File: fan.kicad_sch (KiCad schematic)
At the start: 9 parts, among them J4 Conn_01x04, Q1 BSS138

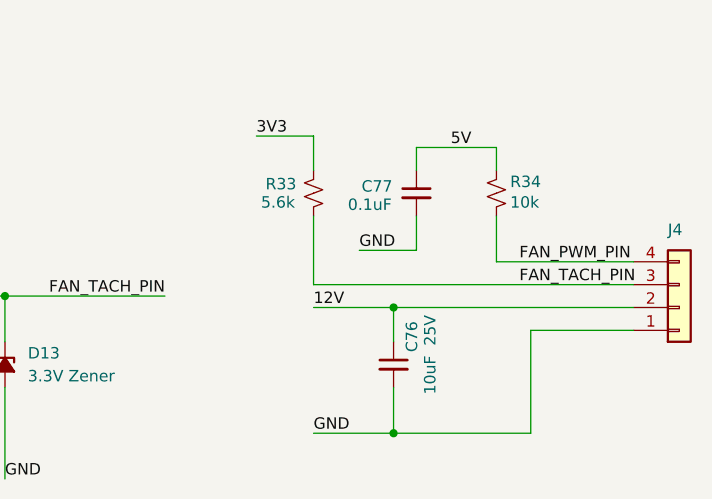
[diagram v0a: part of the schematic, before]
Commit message: run through ERC
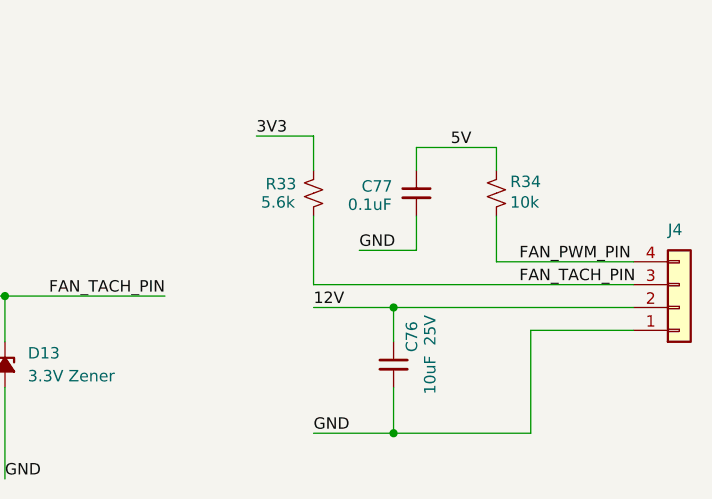
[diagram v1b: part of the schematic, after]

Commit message: adding jlcpcb deets
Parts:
- Q1: FT Rotation Offset (none) -> 180
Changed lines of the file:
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@@
 			)
 		)
-	)
+		(property "FT Rotation Offset" "180"
+			(at 127 92.71 0)
+			(hide yes)
+			(effects
+				(font
+					(size 1.27 1.27)
+				)
+			)
+		))
 	(symbol
 		(lib_id "Device:R_Small_US")
